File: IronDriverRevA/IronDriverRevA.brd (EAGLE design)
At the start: 100 x 100 mm, 46 parts, among them IC1 PIC18F2550, IC2 TL074P, IC3 7805TV, IC4 TL072P, IC5 MC34063AP, Q1 BC557C

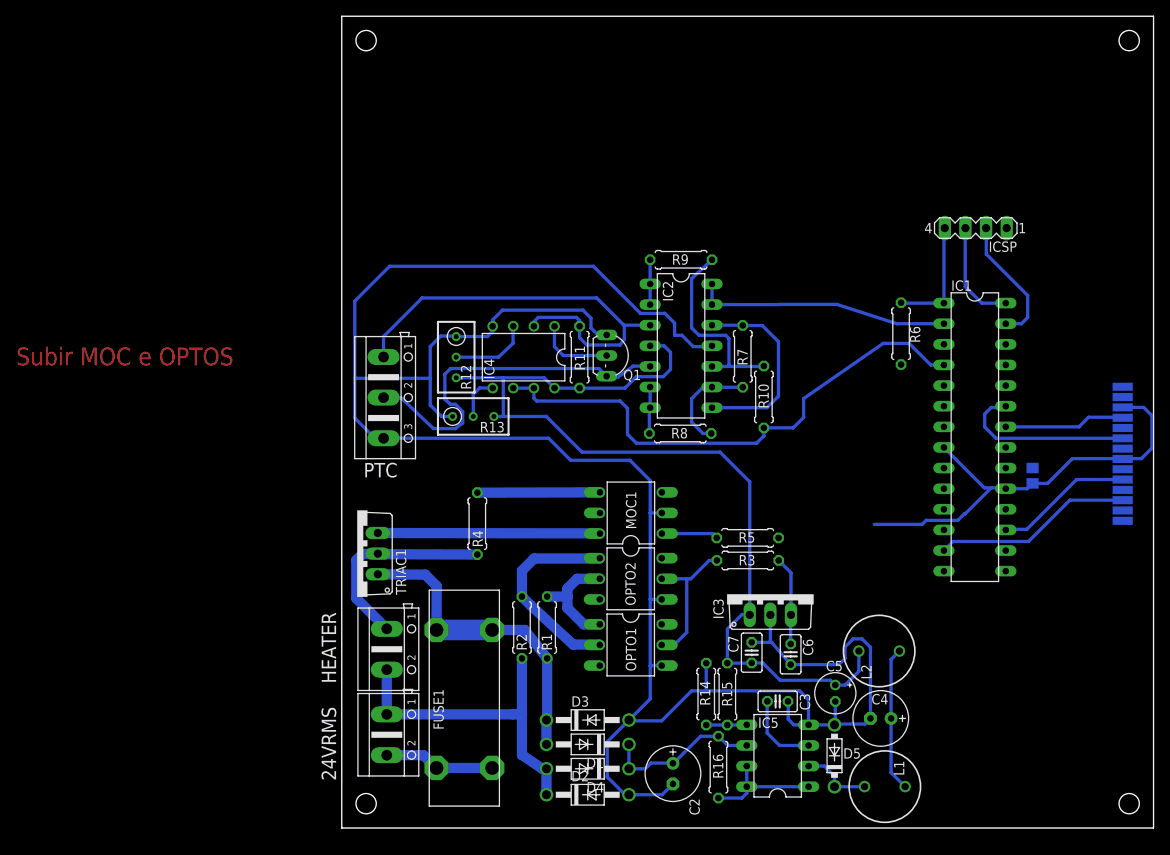
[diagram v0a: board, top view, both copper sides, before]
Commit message: Finalizando Roteamento
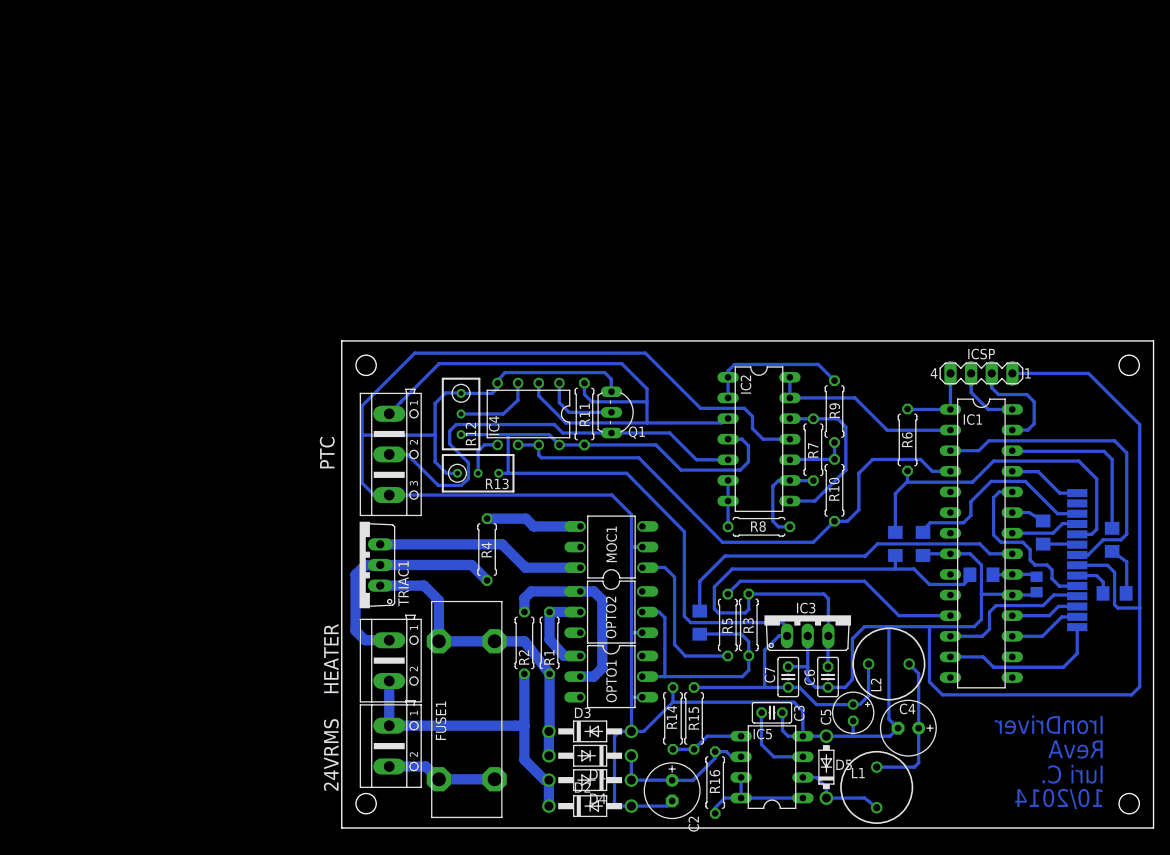
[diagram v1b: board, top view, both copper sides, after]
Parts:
- added JMP1, JMP2, JMP3, JMP4, JMP5, JMP6, JMP7: (no value), rcl:R1206
- moved R9 26.6 mm to (60.7, 51.3), turned to 270 degrees
- moved ICSP 17.9 mm to (78.8, 56.0)
- moved R8 15.0 mm to (51.4, 37.1)
- moved IC2 15.0 mm to (51.4, 47.9)
- moved R10 14.4 mm to (60.7, 41.6)
- moved R7 14.4 mm to (58.1, 46.6)
- moved J1 14.2 mm to (90.6, 33.0)
- moved C1 13.4 mm to (85.6, 30.0)
- moved IC1 13.1 mm to (78.8, 35.0)
- moved R6 13.1 mm to (69.7, 47.8)
- moved R5 11.0 mm to (47.6, 25.0), turned to 270 degrees
- moved R3 7.94 mm to (50.1, 25.0), turned to 90 degrees
- moved PTC 7.03 mm to (5.85, 46.0)
- moved IC4 7.03 mm to (23.0, 51.0)
- moved Q1 7.03 mm to (34.5, 51.2)
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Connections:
- removed net LCD_D4: IC1.3
- removed net LCD_D5: IC1.5
- removed net LCD_D6: IC1.6
- removed net LCD_D7: IC1.7
- new net +5V_JMP4: J1.P$5, JMP4.1, R6.2
- new net +5V_MC: C1.1, IC1.20, JMP3.1
- new net GND_JMP5: J1.P$3, JMP5.1
- new net N$17: J1.P$6, JMP1.2
- new net N$23: J1.P$9, JMP7.2
- new net N$24: JMP6.2, JMP7.1
- new net ZEROCROSSING_B: JMP2.1, OPTO1.5, OPTO2.5, R3.1
- net +5V: now also JMP3.2, JMP4.2; no longer C1.1, IC1.20, J1.P$5, R6.2
- net ENC_B: now also JMP1.1; no longer J1.P$6
- net GND: now also JMP5.2; no longer J1.P$3
- net LCD_BL: now also IC1.25
- net LCD_D0: now also IC1.12
- net LCD_D1: now also IC1.17
- net LCD_D2: now also IC1.3
- net LCD_D3: now also IC1.26, JMP6.1; no longer J1.P$9
- net LCD_E: now also IC1.13; no longer IC1.18
- net LCD_RS: now also IC1.24; no longer IC1.17
- net LCD_RW: now also IC1.18; no longer IC1.13
- net ZEROCROSSING: now also JMP2.2; no longer OPTO1.5, OPTO2.5, R3.1
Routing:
- net GND: track 336.0 -> 413.4 mm
- net +5V: track 10.9 -> 63.3 mm
- net +5V_JMP4: track 0.00 -> 42.4 mm
- net LCD_D2: track 0.00 -> 40.0 mm
- net ZEROCROSSING_B: track 0.00 -> 33.7 mm
- net HEATER: track 0.00 -> 29.9 mm
- net ZEROCROSSING: track 18.1 -> 44.6 mm
- net GND_JMP5: track 0.00 -> 24.4 mm
- net LCD_D3: track 0.00 -> 21.2 mm
- net +PTC: track 55.4 -> 75.7 mm
- net LCD_E: track 0.00 -> 20.2 mm
- net LCD_D0: track 0.00 -> 19.0 mm
- net ENC_B: track 22.2 -> 4.09 mm
- net N$6: track 24.5 -> 7.59 mm
- net LCD_RW: track 24.6 -> 8.48 mm
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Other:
- board size 100 x 100 mm -> 100 x 60 mm
- board text added: "10/2014"
- board text added: "IronDriver"
- board text added: "Iuri C."
- board text added: "RevA"
- board text removed: "Subir MOC e OPTOS"
